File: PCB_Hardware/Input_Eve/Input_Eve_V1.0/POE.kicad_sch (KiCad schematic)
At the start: 23 parts, among them U4 TPS2376D, U5 TX4138, U6 F0505S-2WR2

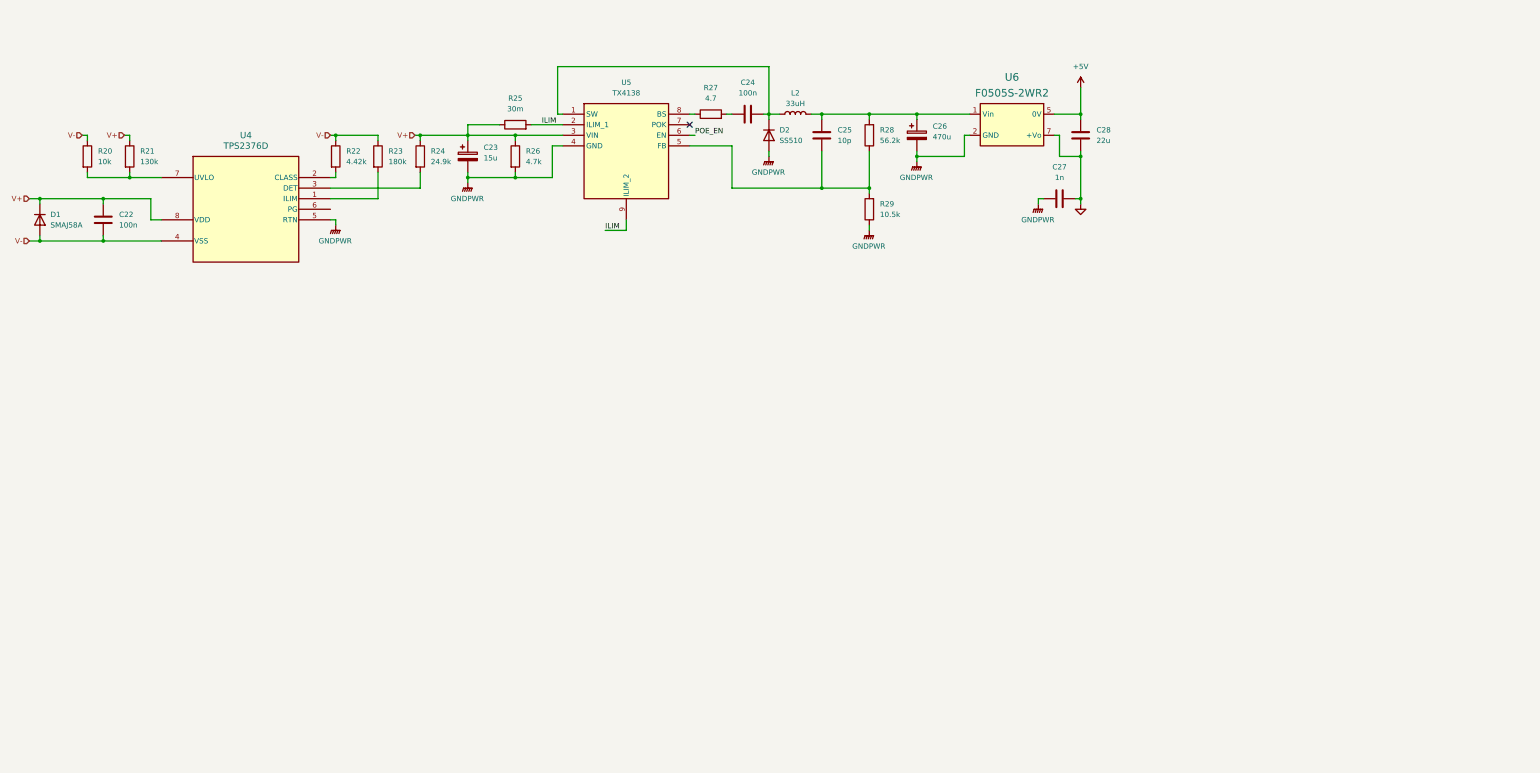
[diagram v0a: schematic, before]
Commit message: Update w new boards/firmware
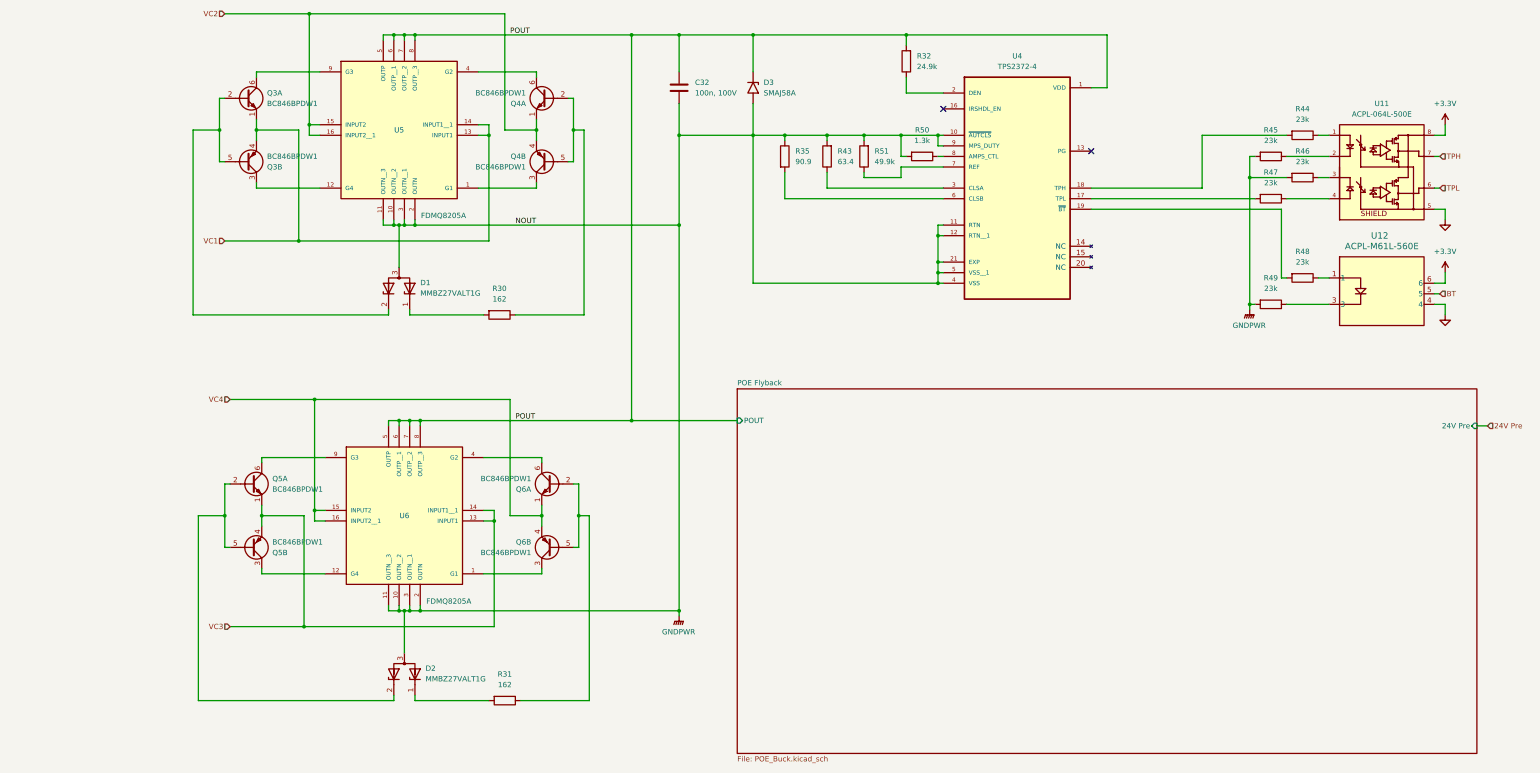
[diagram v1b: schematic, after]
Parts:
- removed C22: 100n, symbol Device:C
- removed C23: 15u, Capacitor_SMD:CP_Elec_10x10.5, symbol Device:C_Polarized
- removed C24: 100n, Capacitor_SMD:C_0402_1005Metric, symbol Device:C
- removed C25: 10p, Capacitor_SMD:C_0402_1005Metric, symbol Device:C
- removed C26: 470u, Capacitor_SMD:CP_Elec_8x10, symbol Device:C_Polarized
- removed C27: 1n, Capacitor_SMD:C_1808_4520Metric, symbol Device:C
- removed C28: 22u, Capacitor_SMD:C_0603_1608Metric, symbol Device:C
- removed D1: SMAJ58A, symbol Device:D
- removed D2: SS510, Diode_SMD:D_SMA, symbol Device:D
- removed L2: 33uH, symbol Device:L
- removed R20: 10k, symbol Device:R
- removed R21: 130k, symbol Device:R
- removed R22: 4.42k, symbol Device:R
- removed R23: 180k, symbol Device:R
- removed R24: 24.9k, symbol Device:R
- removed R25: 30m, Resistor_SMD:R_1206_3216Metric, symbol Device:R
- removed R26: 4.7k, Resistor_SMD:R_2512_6332Metric, symbol Device:R
- removed R27: 4.7, Resistor_SMD:R_0402_1005Metric, symbol Device:R
- removed R28: 56.2k, Resistor_SMD:R_0402_1005Metric, symbol Device:R
- removed R29: 10.5k, Resistor_SMD:R_0402_1005Metric, symbol Device:R
- removed U4: TPS2376D, Package_SO:SOIC-8_3.9x4.9mm_P1.27mm, symbol Tutor_Common_Parts:TPS2376D
- removed U5: TX4138, Package_SO:SOIC-8_3.9x4.9mm_P1.27mm, symbol Tutor_Common_Parts:TX4138
- removed U6: F0505S-2WR2, Tutor_Common_Parts:F0505S-2WR2, symbol Tutor_Common_Parts:F0505S-2WR2
- added C32: 100n, 100V, Capacitor_SMD:C_0805_2012Metric, symbol Device:C
- added D1, D2: MMBZ27VALT1G, Package_TO_SOT_SMD:SOT-23, symbol Diode:MMBZxx
- added D3: SMAJ58A, Diode_SMD:D_SMA, symbol Diode:SMAJ58A
- added Q3, Q4, Q5, Q6: BC846BPDW1, Package_TO_SOT_SMD:SOT-363_SC-70-6, symbol Transistor_BJT:BC846BPDW1
- added R30, R31: 162, Resistor_SMD:R_0402_1005Metric, symbol Device:R
- added R32: 24.9k, Resistor_SMD:R_0402_1005Metric, symbol Device:R
- added R35: 90.9, Resistor_SMD:R_0402_1005Metric, symbol Device:R
- added R43: 63.4, Resistor_SMD:R_0402_1005Metric, symbol Device:R
- added R44, R45, R46, R47, R48, R49: 23k, Resistor_SMD:R_0402_1005Metric, symbol Device:R
- added R50: 1.3k, Resistor_SMD:R_0402_1005Metric, symbol Device:R
- added R51: 49.9k, Resistor_SMD:R_0402_1005Metric, symbol Device:R
- added U11: ACPL-064L-500E, Package_SO:SOIC-8_3.9x4.9mm_P1.27mm, symbol Tutor_Common_Parts:ACPL-064L-500E
- added U12: ACPL-M61L-560E, Tutor_Common_Parts:SO-5_AVA, symbol Tutor_Common_Parts:ACPL-M61L-560E
- added U4: TPS2372-4, Package_DFN_QFN:QFN-20-1EP_5x5mm_P0.65mm_EP3.35x3.35mm, symbol Tutor_Common_Parts:TPS2372-4RGWR
- added U5, U6: FDMQ8205A, Tutor_Common_Parts:FDMQ8205A, symbol Tutor_Common_Parts:FDMQ8205A
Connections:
- net GND: now also U11.5, U12.4
- net GNDPWR: now also C32.2, D1.3 (A), D2.3 (A), D3.2 (A2), R35.1, R43.2, R45.2, R46.2, R49.2, R50.2, R51.2, U4.10 (~{AUTCLS}), U4.11 (RTN), U4.12 (RTN__1), U4.21 (EXP), U4.4 (VSS), U4.5 (VSS__1), U4.9 (MPS_DUTY), U5.10 (OUTN__2), U5.11 (OUTN__3), U5.2 (OUTN), U5.3 (OUTN__1), U6.10 (OUTN__2), U6.11 (OUTN__3), U6.2 (OUTN), U6.3 (OUTN__1)
- new net: R43.1, U4.3 (CLSA)
- new net: Q3.3 (C2), U5.12 (G4)
- new net: D1.2 (K), Q3.2 (B1), Q3.5 (B2)
- new net: Q4.2 (B1), Q4.5 (B2), R30.1
- new net: Q4.6 (C1), U5.4 (G2)
- new net: R44.1, U11.1
- new net: R44.2, U4.18 (TPH)
- new net: R46.1, U11.3
- new net: D1.1 (K), R30.2
- new net: D2.1 (K), R31.2
- new net: D2.2 (K), Q5.2 (B1), Q5.5 (B2)
- new net: R47.1, U11.4
- new net: R47.2, U4.17 (TPL)
- new net: Q4.3 (C2), U5.1 (G1)
- new net: Q3.6 (C1), U5.9 (G3)
- new net: R48.1, U12.1
- new net: R49.1, U12.3
- new net: Q6.3 (C2), U6.1 (G1)
- new net: Q5.3 (C2), U6.12 (G4)
- new net: Q6.6 (C1), U6.4 (G2)
- new net: Q5.6 (C1), U6.9 (G3)
- new net: R48.2, U4.19 (~{BT})
- new net: R32.1, U4.2 (DEN)
- new net: R35.2, U4.6 (CLSB)
- new net: R51.1, U4.7 (REF)
- new net: R50.1, U4.8 (AMPS_CTL)
- new net: R45.1, U11.2
- new net: Q6.2 (B1), Q6.5 (B2), R31.1
- new net +3.3V: U11.8, U12.6
- new net BT: U12.5
- new net POUT: C32.1, D3.1 (A1), R32.2, U4.1 (VDD), U5.5 (OUTP), U5.6 (OUTP__1), U5.7 (OUTP__2), U5.8 (OUTP__3), U6.5 (OUTP), U6.6 (OUTP__1), U6.7 (OUTP__2), U6.8 (OUTP__3)
- new net TPH: U11.7
- new net TPL: U11.6
- new net VC1: Q3.1 (E1), Q3.4 (E2), U5.13 (INPUT1), U5.14 (INPUT1__1)
- new net VC2: Q4.1 (E1), Q4.4 (E2), U5.15 (INPUT2), U5.16 (INPUT2__1)
- new net VC3: Q5.1 (E1), Q5.4 (E2), U6.13 (INPUT1), U6.14 (INPUT1__1)
- new net VC4: Q6.1 (E1), Q6.4 (E2), U6.15 (INPUT2), U6.16 (INPUT2__1)
- no-connect marks 1 -> 2
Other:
- added sheet POE Flyback (POE_Buck.kicad_sch)
